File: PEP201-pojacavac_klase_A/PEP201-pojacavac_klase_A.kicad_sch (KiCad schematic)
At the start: 18 parts, among them J1 Screw_Terminal_01x02, J2 Conn_01x02_Pin, J3 Conn_01x02_Pin, J4 Conn_01x02_Pin, J5 Conn_01x02_Pin, Q1 MMBT2222A

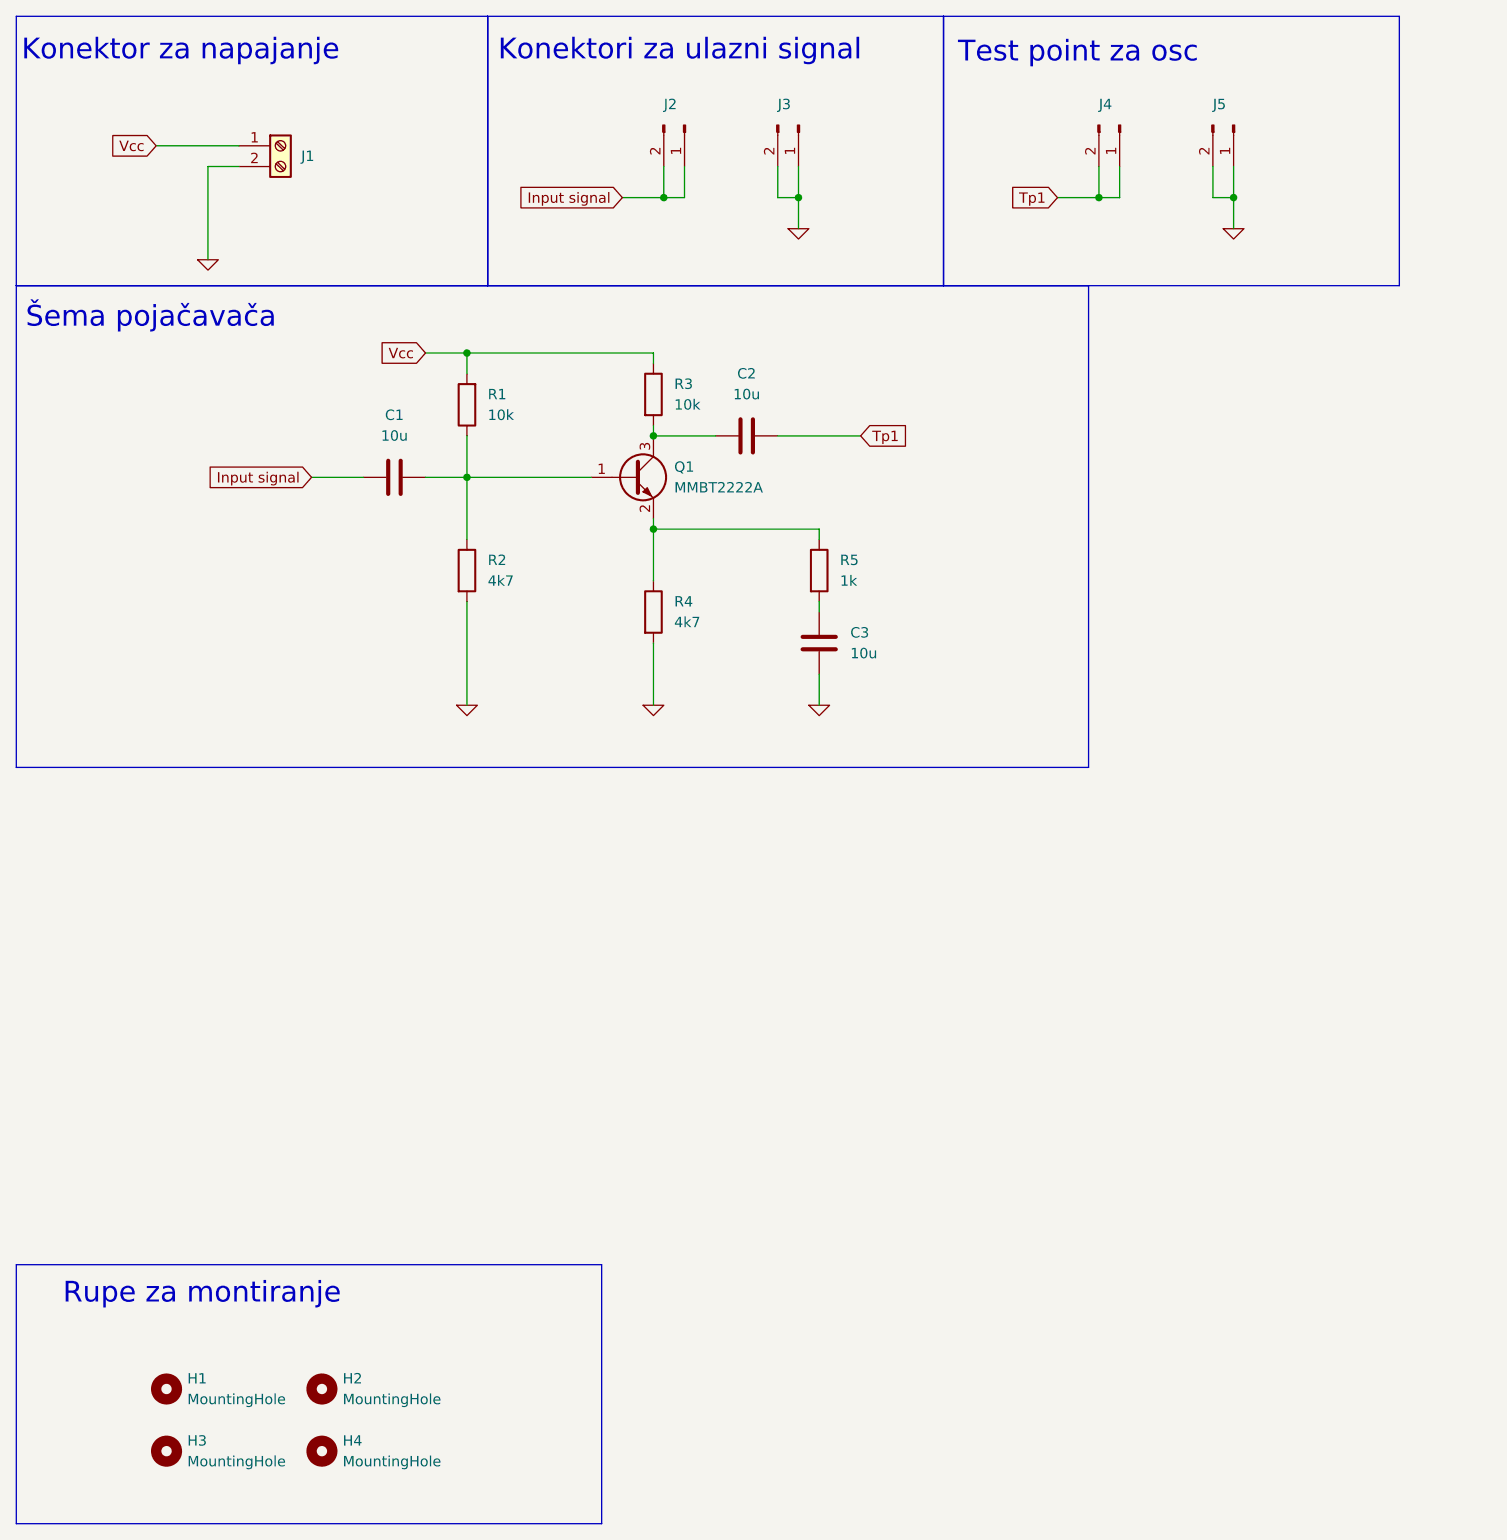
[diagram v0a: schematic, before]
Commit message: Nova estetika.
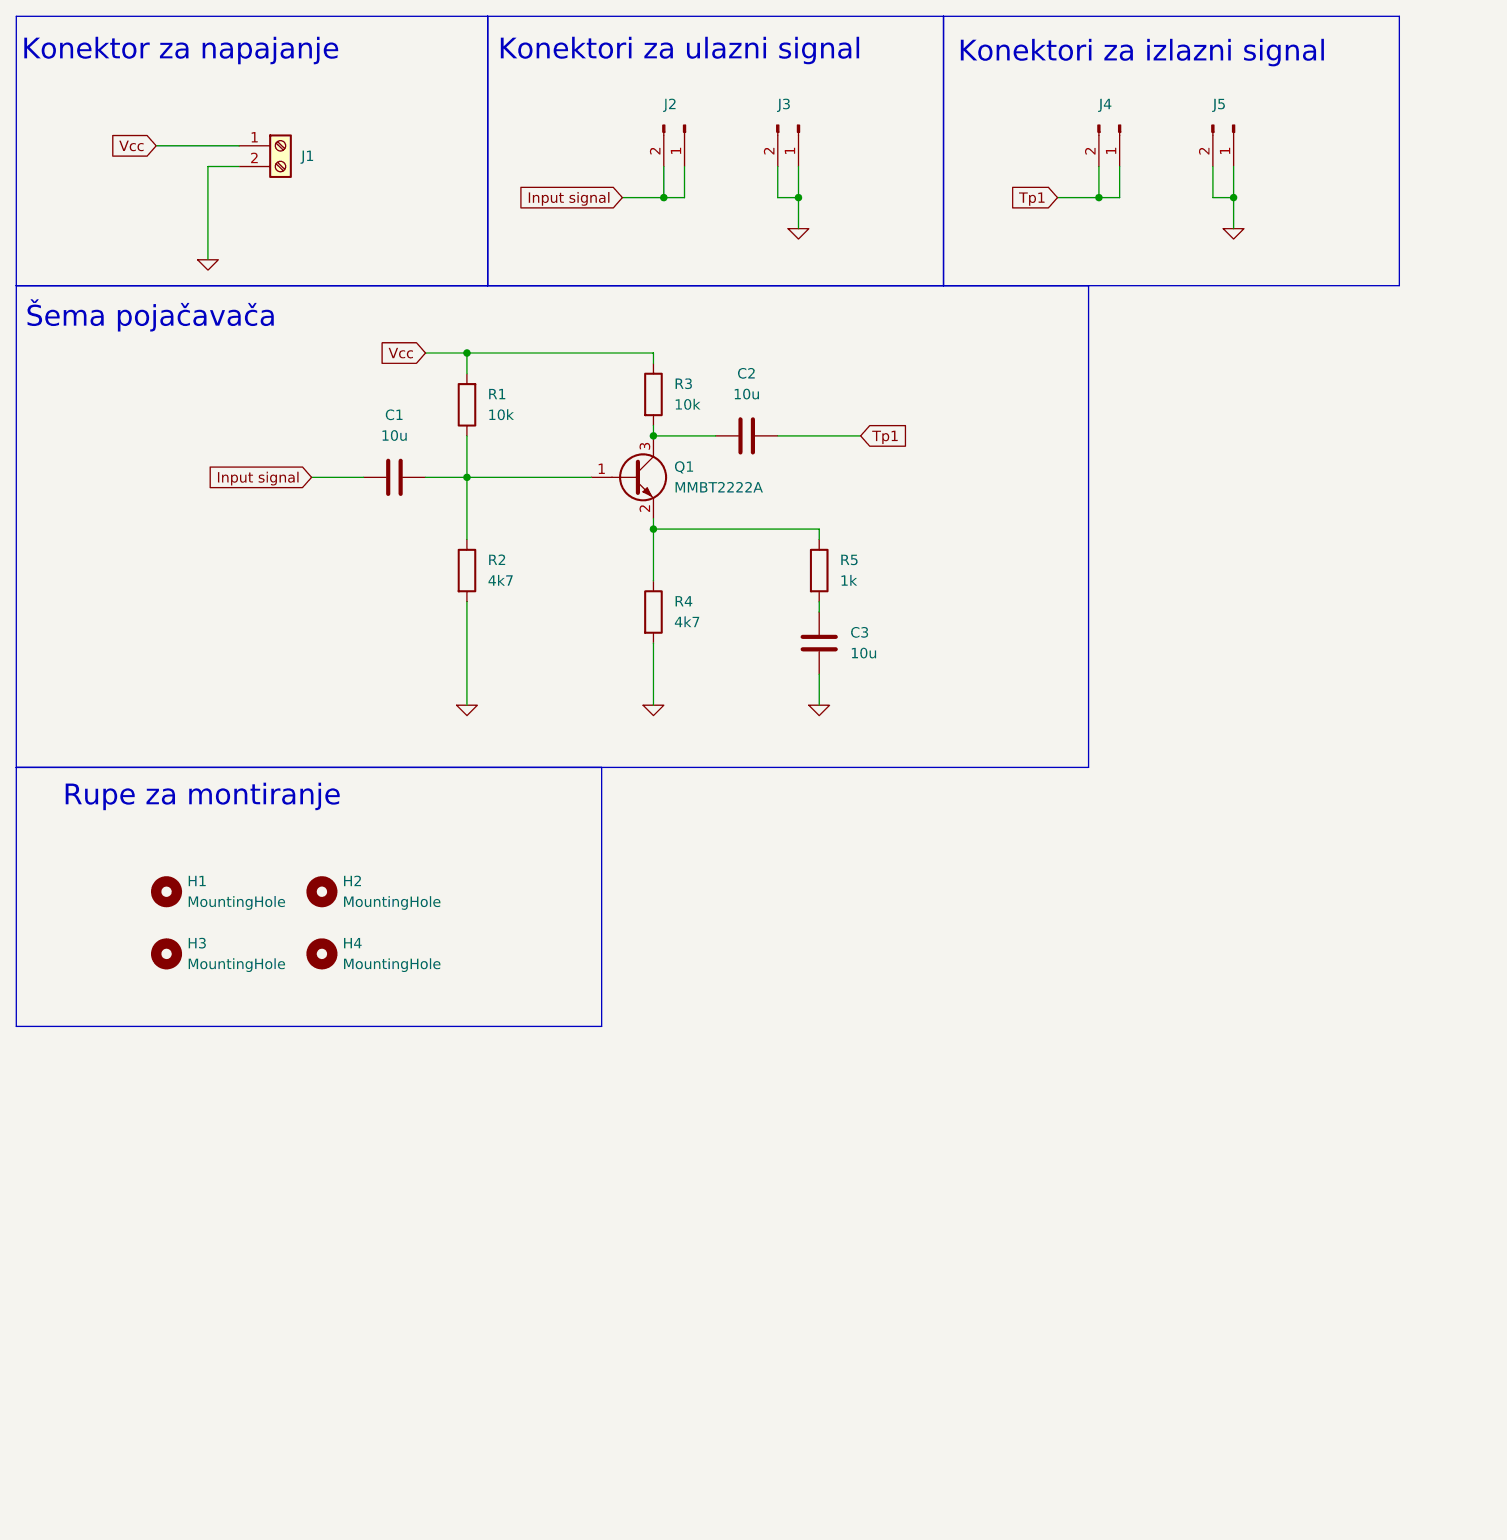
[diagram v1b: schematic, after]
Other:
- note added: "Konektori za izlazni signal"
- note removed: "Test point za osc"
- moved on the sheet: H1, H2, H3, H4
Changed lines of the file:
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@@
 	(generator "eeschema")
 	(generator_version "9.0")
-	(paper "A4")
+	(paper "A5")
 	(title_block
 		(title "Pojačavač klase A")
@@
 	)
 	(rectangle
-		(start 12.065 165.1)
-		(end 83.82 196.85)
+		(start 12.065 104.14)
+		(end 83.82 135.89)
 		(stroke
 			(width 0)
@@
 	(text "Rupe za montiranje\n"
 		(exclude_from_sim no)
-		(at 17.78 170.18 0)
+		(at 17.78 109.22 0)
 		(effects
 			(font
@@
 		)
 	)
-	(text "Test point za osc"
+	(text "Konektori za izlazni signal"
 		(exclude_from_sim no)
 		(at 127.508 18.034 0)
@@
 	(symbol
 		(lib_id "Mechanical:MountingHole")
-		(at 30.48 187.96 0)
+		(at 30.48 127 0)
 		(unit 1)
 		(exclude_from_sim no)
@@
 		(fields_autoplaced yes)
 		(property "Reference" "H3"
-			(at 33.02 186.69 0)
+			(at 33.02 125.73 0)
 			(effects
 				(font
@@
 		)
 		(property "Value" "MountingHole"
-			(at 33.02 189.23 0)
+			(at 33.02 128.27 0)
 			(effects
 				(font
@@
 		)
 		(property "Footprint" "MountingHole:MountingHole_3.2mm_M3_ISO14580_Pad_TopBottom"
-			(at 30.48 187.96 0)
+			(at 30.48 127 0)
 			(effects
 				(font
@@
 		)
 		(property "Datasheet" "~"
-			(at 30.48 187.96 0)
+			(at 30.48 127 0)
 			(effects
 				(font
@@
 		)
 		(property "Description" ""
-			(at 30.48 187.96 0)
+			(at 30.48 127 0)
 			(effects
 				(font
@@
 	(symbol
 		(lib_id "Mechanical:MountingHole")
-		(at 49.53 180.34 0)
+		(at 49.53 119.38 0)
 		(unit 1)
 		(exclude_from_sim no)
@@
 		(fields_autoplaced yes)
 		(property "Reference" "H2"
-			(at 52.07 179.07 0)
+			(at 52.07 118.11 0)
 			(effects
 				(font
@@
 		)
 		(property "Value" "MountingHole"
-			(at 52.07 181.61 0)
+			(at 52.07 120.65 0)
 			(effects
 				(font
@@
 		)
 		(property "Footprint" "MountingHole:MountingHole_3.2mm_M3_ISO14580_Pad_TopBottom"
-			(at 49.53 180.34 0)
+			(at 49.53 119.38 0)
 			(effects
 				(font
@@
 		)
 		(property "Datasheet" "~"
-			(at 49.53 180.34 0)
+			(at 49.53 119.38 0)
 			(effects
 				(font
@@
 		)
 		(property "Description" ""
-			(at 49.53 180.34 0)
+			(at 49.53 119.38 0)
 			(effects
 				(font
@@
 	(symbol
 		(lib_id "Mechanical:MountingHole")
-		(at 30.48 180.34 0)
+		(at 30.48 119.38 0)
 		(unit 1)
 		(exclude_from_sim no)
@@
 		(fields_autoplaced yes)
 		(property "Reference" "H1"
-			(at 33.02 179.07 0)
+			(at 33.02 118.11 0)
 			(effects
 				(font
@@
 		)
 		(property "Value" "MountingHole"
-			(at 33.02 181.61 0)
+			(at 33.02 120.65 0)
 			(effects
 				(font
@@
 		)
 		(property "Footprint" "MountingHole:MountingHole_3.2mm_M3_ISO14580_Pad_TopBottom"
-			(at 30.48 180.34 0)
+			(at 30.48 119.38 0)
 			(effects
 				(font
@@
 		)
 		(property "Datasheet" "~"
-			(at 30.48 180.34 0)
+			(at 30.48 119.38 0)
 			(effects
 				(font
@@
 		)
 		(property "Description" ""
-			(at 30.48 180.34 0)
+			(at 30.48 119.38 0)
 			(effects
 				(font
@@
 	(symbol
 		(lib_id "Mechanical:MountingHole")
-		(at 49.53 187.96 0)
+		(at 49.53 127 0)
 		(unit 1)
 		(exclude_from_sim no)
@@
 		(fields_autoplaced yes)
 		(property "Reference" "H4"
-			(at 52.07 186.69 0)
+			(at 52.07 125.73 0)
 			(effects
 				(font
@@
 		)
 		(property "Value" "MountingHole"
-			(at 52.07 189.23 0)
+			(at 52.07 128.27 0)
 			(effects
 				(font
@@
 		)
 		(property "Footprint" "MountingHole:MountingHole_3.2mm_M3_ISO14580_Pad_TopBottom"
-			(at 49.53 187.96 0)
+			(at 49.53 127 0)
 			(effects
 				(font
@@
 		)
 		(property "Datasheet" "~"
-			(at 49.53 187.96 0)
+			(at 49.53 127 0)
 			(effects
 				(font
@@
 		)
 		(property "Description" ""
-			(at 49.53 187.96 0)
-			(effects
-				(font
+			(at 49.53 127 0)
+			(effects
+				(font
